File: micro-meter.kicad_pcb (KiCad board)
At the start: 2 copper layers, 144 parts, among them J1 DC_IN, J10 5V_OUT, J11 LEDS_DATA, J12 LEDS_EXT, J2 SPI, J3 I2C / UART, J4 IN1, J5 IN2, J6 IN3, J7 IN4, J8 SWD, J9 USB_B_Micro, U1 MP2359, U2 STM32F411CEU6, U3 XC6206P332MR, U4 MCP6002-ISN, Y1 16MHz

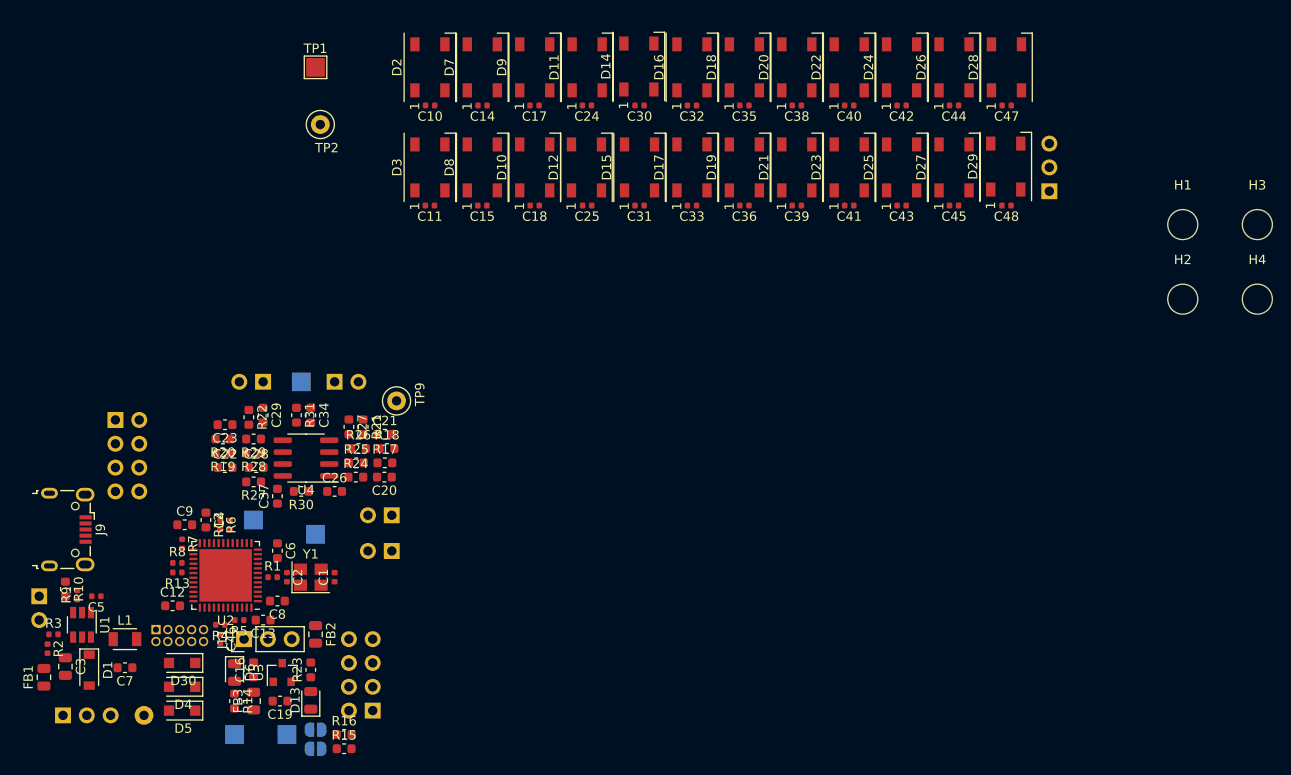
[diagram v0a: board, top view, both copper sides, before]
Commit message: Cleanup layout
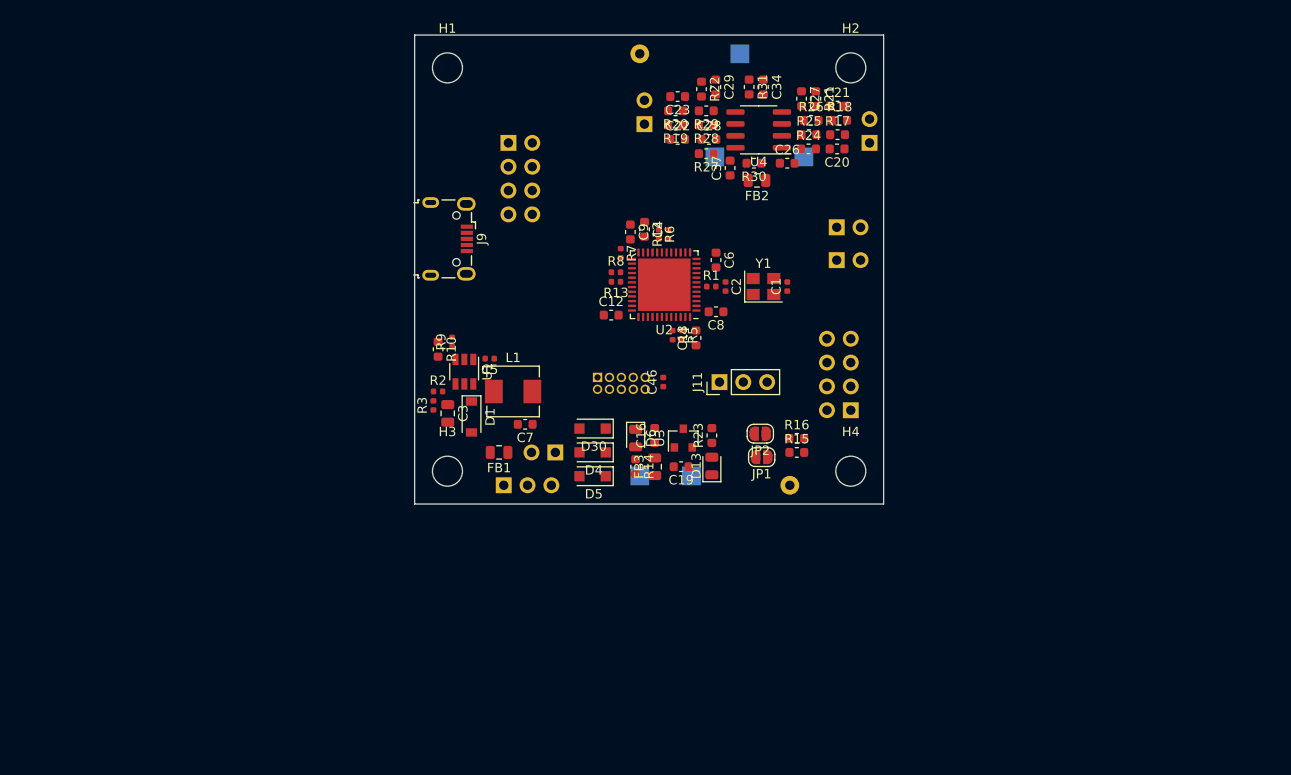
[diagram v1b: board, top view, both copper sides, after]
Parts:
- removed C10, C11, C14, C15, C17, C18, C24, C25, C30, C31, C32, C33, C35, C36, C38, C39, C40, C41, C42, C43, C44, C45, C47, C48: 0.1u, Capacitor_SMD:C_0402_1005Metric
- removed D10, D11, D12, D14, D15, D16, D17, D18, D19, D2, D20, D21, D22, D23, D24, D25, D26, D27, D28, D29, D3, D7, D8, D9: WS2812C, LED_SMD:LED_WS2812B_PLCC4_5.0x5.0mm_P3.2mm
- removed J12: LEDS_EXT, Connector_PinHeader_2.54mm:PinHeader_1x03_P2.54mm_Vertical
- removed TP1: TP_DIN, TestPoint:TestPoint_Pad_2.0x2.0mm
- removed TP2: TP_GND, TestPoint:TestPoint_Loop_D2.50mm_Drill1.0mm
- JP1, JP2: moved to F.Cu
- L1: footprint Inductor_SMD:L_TDK_NLV25_2.5x2.0mm -> Inductor_SMD:L_Sunlord_MWSA0518_5.4x5.2mm
- TP9: moved to B.Cu
- moved H3 90.3 mm to (73.5, 166.5)
- moved H1 80.2 mm to (73.5, 123.5)
- moved TP5 73.1 mm to (110.0, 168.0)
- moved FB2 67.5 mm to (106.5, 135.5), turned to 180 degrees
- moved TP6 65.8 mm to (111.5, 133.0)
- moved TP7 62.6 mm to (102.0, 133.0)
- moved J4 62.5 mm to (118.5, 131.5), turned to 0 degrees
- moved J3 60.2 mm to (116.5, 160.0)
- moved C22 59.6 mm to (98.0, 131.1)
- moved C28 59.6 mm to (101.4, 131.1)
- moved C20 59.6 mm to (115.0, 132.1)
- moved C21 59.6 mm to (115.1, 127.6)
- moved C23 59.6 mm to (98.0, 126.6)
- moved C27 59.6 mm to (111.3, 126.8)
- moved C37 59.6 mm to (103.6, 134.2)
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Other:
- board outline added: 50 x 50 mm
